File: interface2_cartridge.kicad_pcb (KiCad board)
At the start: 2 copper layers, 38.1 x 38.1 mm, 13 parts, among them J1 cartridge_IF2, J2 Conn_01x05, U1 29F010-TSOP-SP

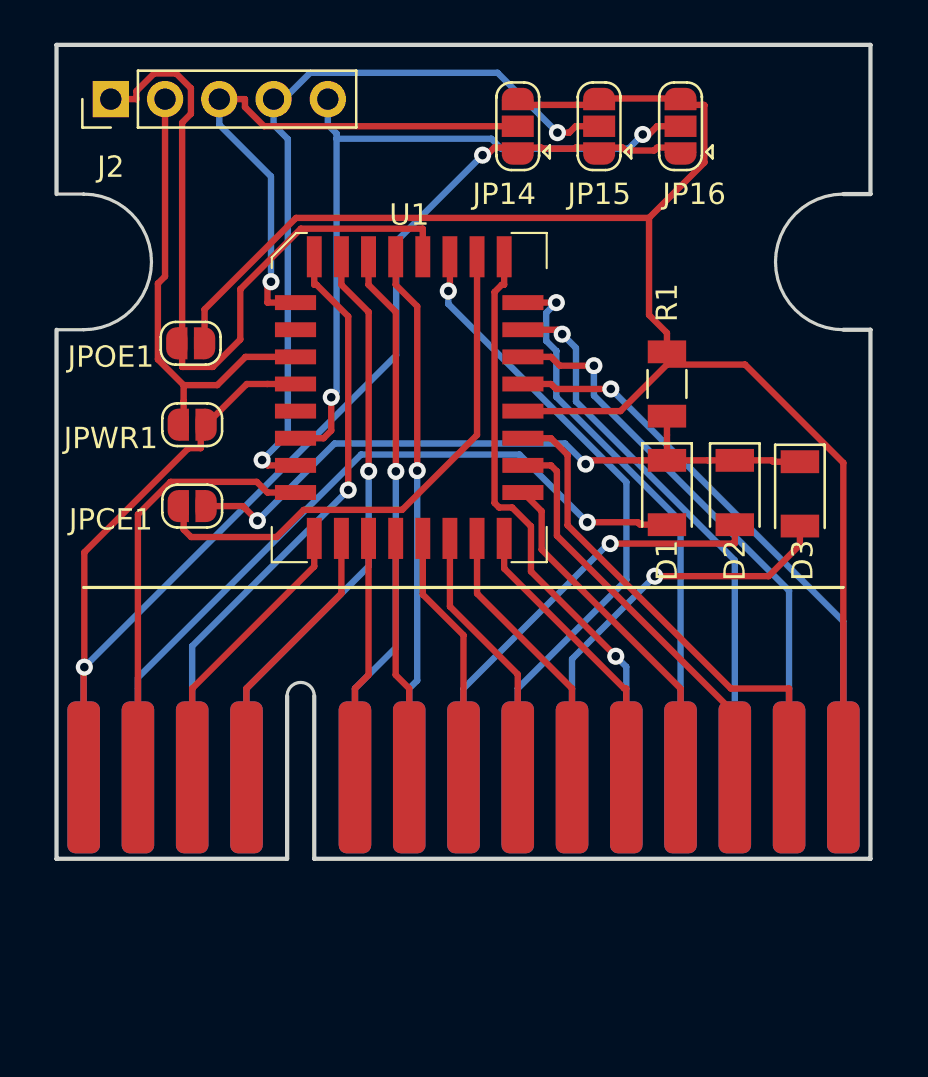
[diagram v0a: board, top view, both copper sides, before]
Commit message: final design
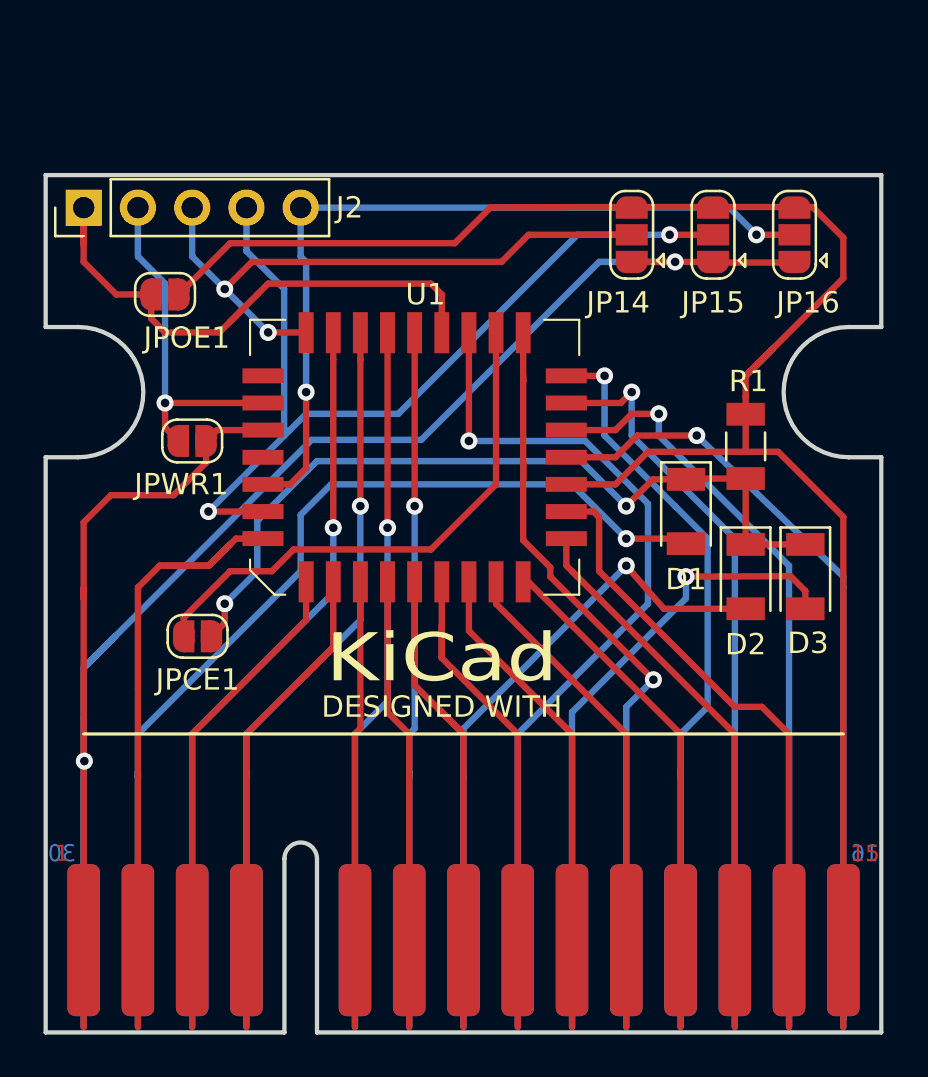
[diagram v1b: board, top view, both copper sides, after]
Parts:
- U1: value 29F010-TSOP-SP -> AM29F010B; footprint Package_LCC:PLCC-32 -> SINCLAIR:PLCC-32
- moved J1 7.62 mm to (124.5, 91.4)
- moved JP14 7.37 mm to (140.0, 58.4)
- moved JP15 7.37 mm to (143.8, 58.4)
- moved JP16 7.37 mm to (147.6, 58.4)
- moved JPCE1 6.10 mm to (119.6, 77.2)
- moved J2 5.24 mm to (114.3, 57.1)
- moved R1 4.70 mm to (145.3, 68.3)
- moved D2 3.97 mm to (145.3, 74.4)
- moved D3 3.88 mm to (148.1, 74.4)
- moved U1 2.81 mm to (129.8, 68.8), turned to 90 degrees
- moved JPOE1 2.58 mm to (118.1, 61.2)
- moved D1 1.26 mm to (142.5, 71.4)
- moved JPWR1 0.76 mm to (119.4, 68.1)
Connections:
- U1 pad 1: A11 -> (no net)
- U1 pad 10: A16 -> A2
- U1 pad 11: A15 -> A1
- U1 pad 12: A12 -> A0
- U1 pad 13: A7 -> D0
- U1 pad 14: A6 -> D1
- U1 pad 15: A5 -> D2
- U1 pad 16: A4 -> GND
- U1 pad 17: A3 -> D3
- U1 pad 18: A2 -> D4
- U1 pad 19: A1 -> D5
- U1 pad 2: A9 -> A16
- U1 pad 20: A0 -> D6
- U1 pad 21: D0 -> D7
- U1 pad 22: D1 -> Net-(JPCE1-Pad1)
- U1 pad 23: D2 -> A10
- U1 pad 24: GND -> Net-(J2-Pad1)
- U1 pad 25: D3 -> A11
- U1 pad 26: D4 -> A9
- U1 pad 27: D5 -> A8
- U1 pad 28: D6 -> A13
- U1 pad 29: D7 -> A14
- U1 pad 3: A8 -> A15
- U1 pad 30: Net-(JPCE1-Pad1) -> (no net)
- U1 pad 31: A10 -> Net-(J2-Pad2)
- U1 pad 32: Net-(J2-Pad1) -> +5V
- U1 pad 4: A13 -> A12
- U1 pad 5: A14 -> A7
- U1 pad 6: (no net) -> A6
- U1 pad 7: Net-(J2-Pad2) -> A5
- U1 pad 8: +5V -> A4
- U1 pad 9: (no net) -> A3
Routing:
- net +5V: track 71.8 -> 95.7 mm
- net A1: track 13.0 -> 24.2 mm
- net D3: track 26.9 -> 36.7 mm
- net A6: track 13.0 -> 21.7 mm
- net Net-(J2-Pad1): track 34.9 -> 26.7 mm
- net Net-(D1-Pad2): track 35.1 -> 43.1 mm
- net A3: track 12.0 -> 19.6 mm
- net A2: track 12.5 -> 20.0 mm
- net A10: track 30.0 -> 37.1 mm
- net Net-(D3-Pad2): track 19.3 -> 25.9 mm
- net Net-(D2-Pad2): track 20.6 -> 27.2 mm
- net A15: track 36.4 -> 42.9 mm
- net A12: track 20.5 -> 27.0 mm
- net A4: track 11.5 -> 17.7 mm
- net A0: track 13.6 -> 19.3 mm
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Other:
- board size 38.1 x 38.1 mm -> 39.1 x 40.1 mm
- board text added: "1"
- board text added: "15"
- board text added: "16"
- board text added: "30"
- board text added: "8 Banks of 16Kb, Also compatible with Dandanator 2.0 VC"
- board text added: "DESIGNED WITH"
- board text added: "KiCad"
- board text removed: "8 Banks of 16Kb, Also compatible with Dandanator VC 2.0"
